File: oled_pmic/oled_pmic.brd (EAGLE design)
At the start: 16.5 x 16 mm, 11 parts, among them J1 I_sense, J2 VCC, J4 GND, Q1 N-CHANNEL-MOSFETSOT23-3, U1 AL5801W6-7

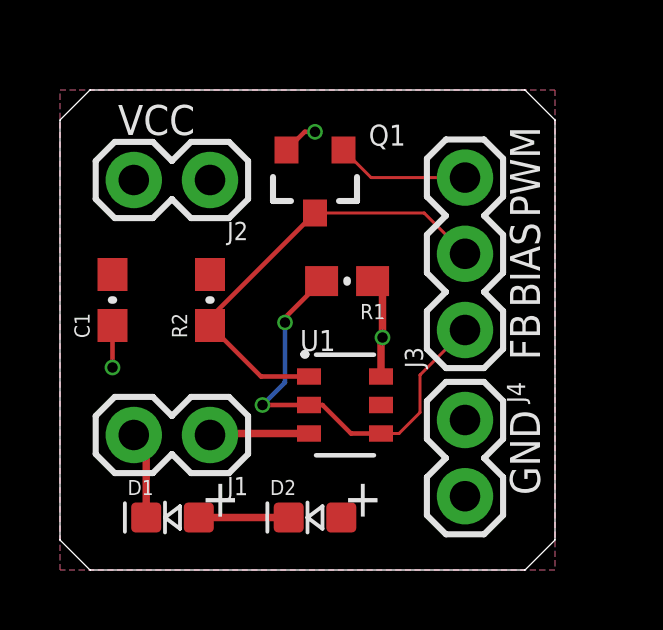
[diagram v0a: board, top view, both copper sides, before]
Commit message: place order
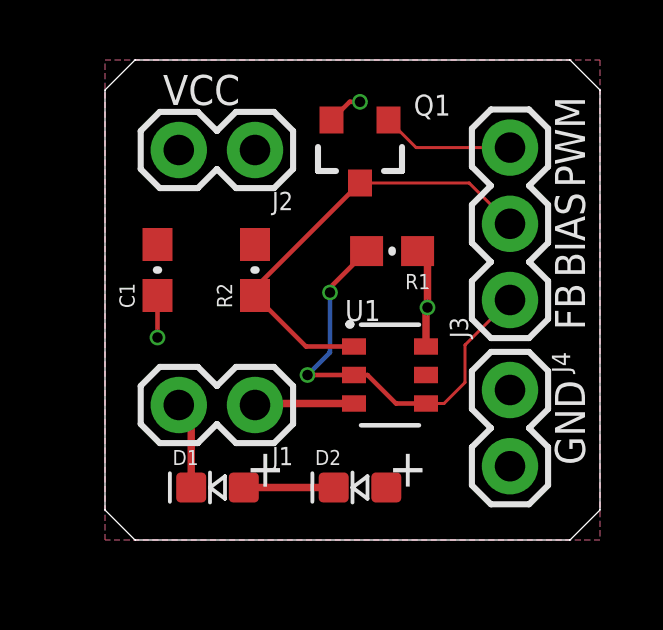
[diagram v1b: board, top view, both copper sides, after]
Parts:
- moved C1 1.80 mm to (1.75, 9.00)
- moved D1 1.80 mm to (3.75, 1.75)
- moved D2 1.80 mm to (8.50, 1.75)
- moved J1 1.80 mm to (5.00, 4.50)
- moved J2 1.80 mm to (5.00, 13.0)
- moved J3 1.80 mm to (13.5, 8.00)
- moved J4 1.80 mm to (13.5, 5.00)
- moved Q1 1.80 mm to (8.50, 13.0)
- moved R1 1.80 mm to (9.57, 9.63)
- moved R2 1.80 mm to (5.00, 9.00)
- moved U1 1.80 mm to (9.50, 5.50)
